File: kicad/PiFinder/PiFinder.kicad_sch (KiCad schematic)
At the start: 24 parts, among them J1 Raspberry_Pi_2_3, J2 display, J3 IMU, SW0 SW_Push_Dual, SW1 SW_Push_Dual, SW2 SW_Push_Dual, SW3 SW_Push_Dual, SW4 SW_Push_Dual, SW5 SW_Push_Dual, SW6 SW_Push_Dual, SW7 SW_Push_Dual, SW8 SW_Push_Dual, SW9 SW_Push_Dual

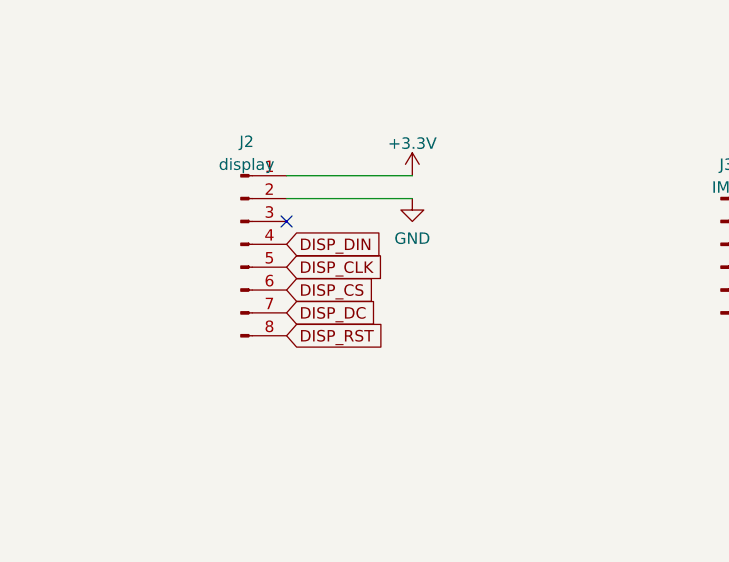
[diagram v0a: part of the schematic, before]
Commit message: Working capture/solver
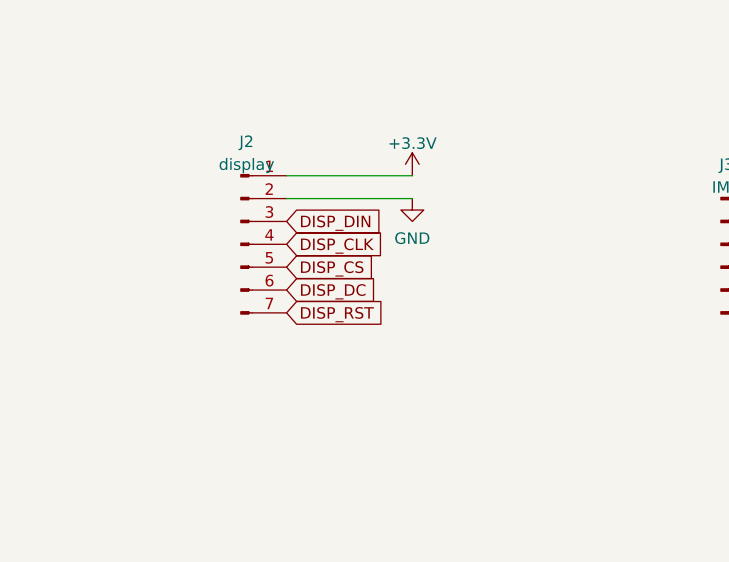
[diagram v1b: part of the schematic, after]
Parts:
- J2: symbol Connector:Conn_01x08_Male -> Connector:Conn_01x07_Male
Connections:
- net DISP_CLK: now also J2.4 (Pin_4); no longer J2.5 (Pin_5)
- net DISP_CS: now also J2.5 (Pin_5); no longer J2.6 (Pin_6)
- net DISP_DC: now also J2.6 (Pin_6); no longer J2.7 (Pin_7)
- net DISP_DIN: now also J2.3 (Pin_3); no longer J2.4 (Pin_4)
- net DISP_RST: now also J2.7 (Pin_7); no longer J2.8 (Pin_8)
- no-connect marks 3 -> 2
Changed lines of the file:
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@@
   (junction (at 46.99 180.34) (diameter 0) (color 0 0 0 0)
   )
-  (no_connect (at 45.72 43.18))
   (no_connect (at 99.06 53.34))
   (no_connect (at 99.06 43.18))
@@
     )
   )
-  (global_label "DISP_DC" (shape input) (at 45.72 53.34 0) (fields_autoplaced)
-    (effects (font (size 1.27 1.27)) (justify left))
-    (property "Intersheet References" "${INTERSHEET_REFS}" (id 0) (at 55.9061 53.2606 0)
+  (global_label "DISP_DC" (shape input) (at 45.72 50.8 0) (fields_autoplaced)
+    (effects (font (size 1.27 1.27)) (justify left))
+    (property "Intersheet References" "${INTERSHEET_REFS}" (id 0) (at 55.9061 50.7206 0)
       (effects (font (size 1.27 1.27)) (justify left) hide)
     )
@@
     )
   )
-  (global_label "DISP_RST" (shape input) (at 45.72 55.88 0) (fields_autoplaced)
-    (effects (font (size 1.27 1.27)) (justify left))
-    (property "Intersheet References" "${INTERSHEET_REFS}" (id 0) (at 56.8132 55.8006 0)
-      (effects (font (size 1.27 1.27)) (justify left) hide)
-    )
-  )
-  (global_label "DISP_CLK" (shape input) (at 45.72 48.26 0) (fields_autoplaced)
-    (effects (font (size 1.27 1.27)) (justify left))
-    (property "Intersheet References" "${INTERSHEET_REFS}" (id 0) (at 56.9342 48.1806 0)
-      (effects (font (size 1.27 1.27)) (justify left) hide)
-    )
-  )
-  (global_label "DISP_CS" (shape input) (at 45.72 50.8 0) (fields_autoplaced)
-    (effects (font (size 1.27 1.27)) (justify left))
-    (property "Intersheet References" "${INTERSHEET_REFS}" (id 0) (at 55.8456 50.7206 0)
+  (global_label "DISP_RST" (shape input) (at 45.72 53.34 0) (fields_autoplaced)
+    (effects (font (size 1.27 1.27)) (justify left))
+    (property "Intersheet References" "${INTERSHEET_REFS}" (id 0) (at 56.8132 53.2606 0)
+      (effects (font (size 1.27 1.27)) (justify left) hide)
+    )
+  )
+  (global_label "DISP_CLK" (shape input) (at 45.72 45.72 0) (fields_autoplaced)
+    (effects (font (size 1.27 1.27)) (justify left))
+    (property "Intersheet References" "${INTERSHEET_REFS}" (id 0) (at 56.9342 45.6406 0)
+      (effects (font (size 1.27 1.27)) (justify left) hide)
+    )
+  )
+  (global_label "DISP_CS" (shape input) (at 45.72 48.26 0) (fields_autoplaced)
+    (effects (font (size 1.27 1.27)) (justify left))
+    (property "Intersheet References" "${INTERSHEET_REFS}" (id 0) (at 55.8456 48.1806 0)
       (effects (font (size 1.27 1.27)) (justify left) hide)
     )
@@
     )
   )
-  (global_label "DISP_DIN" (shape input) (at 45.72 45.72 0) (fields_autoplaced)
-    (effects (font (size 1.27 1.27)) (justify left))
-    (property "Intersheet References" "${INTERSHEET_REFS}" (id 0) (at 56.5713 45.6406 0)
+  (global_label "DISP_DIN" (shape input) (at 45.72 43.18 0) (fields_autoplaced)
+    (effects (font (size 1.27 1.27)) (justify left))
+    (property "Intersheet References" "${INTERSHEET_REFS}" (id 0) (at 56.5713 43.1006 0)
       (effects (font (size 1.27 1.27)) (justify left) hide)
     )
@@
     (pin "1")
   )
-  (symbol (lib_id "Connector:Conn_01x08_Male") (at 40.64 45.72 0) (unit 1)
+  (symbol (lib_id "Connector:Conn_01x07_Male") (at 40.64 45.72 0) (unit 1)
     (in_bom yes) (on_board yes) (fields_autoplaced)
     (property "Reference" "J2" (id 0) (at 41.275 34.324 0))
@@
     (pin "6")
     (pin "7")
-    (pin "8")
   )
   (symbol (lib_id "power:GND") (at 59.69 40.64 0) (unit 1)
